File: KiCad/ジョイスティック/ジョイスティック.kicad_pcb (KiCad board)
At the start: 2 copper layers, 30 x 30 mm, 3 parts, among them J1 Conn_01x05_Pin

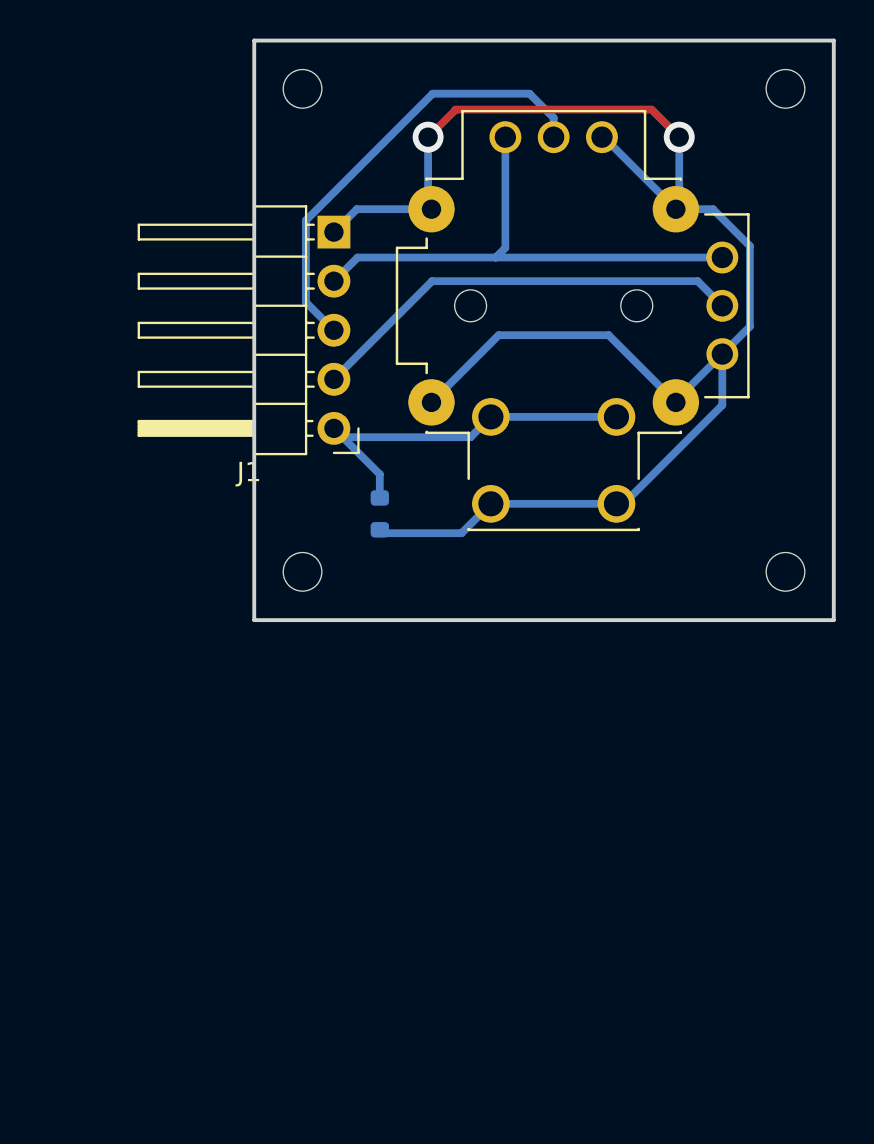
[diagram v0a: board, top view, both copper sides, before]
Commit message: バカの配線を破壊
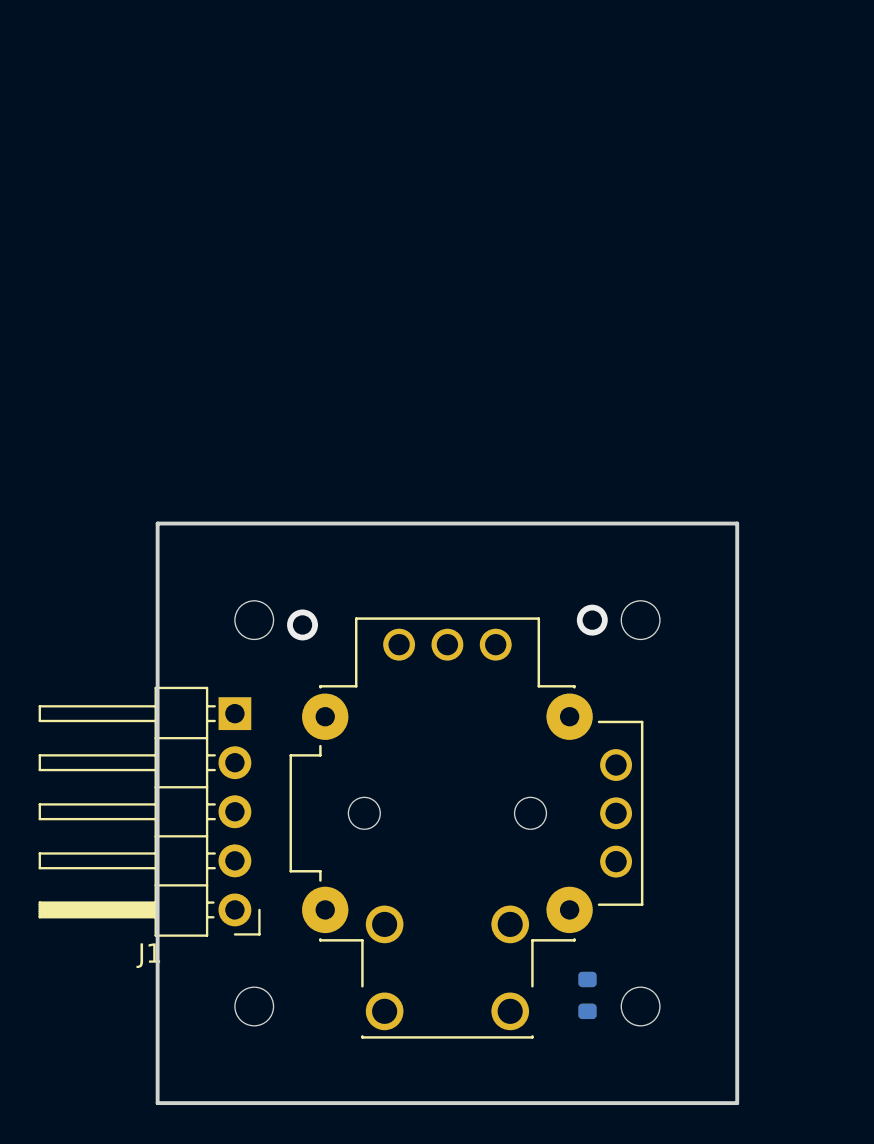
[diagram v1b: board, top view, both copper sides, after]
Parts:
- moved R1 27.1 mm to (127.2, 129.4), turned to 90 degrees
- moved S1 26.8 mm to (120.0, 120.0)
- moved J1 25.4 mm to (109.0, 125.0)
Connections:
- R1 pad 2: GND -> /Vin
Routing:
- net GND: track 85.5 -> 0.00 mm
- net /Vin: track 27.0 -> 0.00 mm
- net /VR2: track 23.3 -> 0.00 mm
- net /VR1: track 22.7 -> 0.00 mm
- net /SW: track 19.9 -> 0.00 mm
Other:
- outline, holes or cut-outs redrawn
